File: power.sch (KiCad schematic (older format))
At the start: 18 parts, among them Q1 BSS84, Q2 BSS138, SW1 TL3342, U3 NCP1402SN33T1G

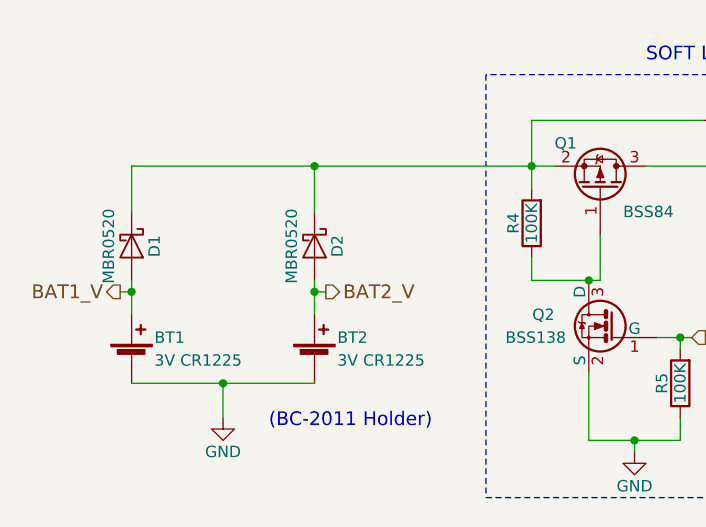
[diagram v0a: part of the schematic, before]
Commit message: attempt 1
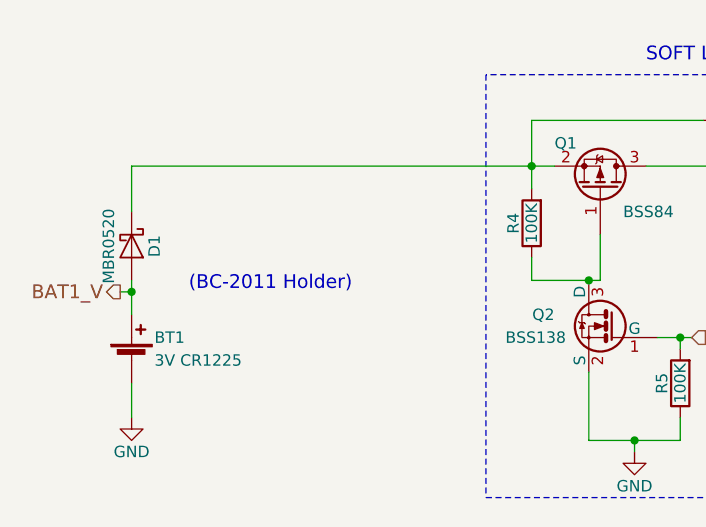
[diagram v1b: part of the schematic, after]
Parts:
- removed BT2: 3V CR1225, BC_2011_CR1225_HOLDER:BC-2011-CR1225, symbol Battery_Cell
- removed D2: MBR0520, Diodes_SMD:D_SOD-123, symbol MBR0520
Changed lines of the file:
@@
-	1    0    0    -1
-$EndComp
-$Comp
-L Battery_Cell BT2
-U 1 1 59A123DB
-P 2300 4050
-F 0 "BT2" H 2400 4150 50  0000 L CNN
-F 1 "3V CR1225" H 2400 4050 50  0000 L CNN
-F 2 "BC_2011_CR1225_HOLDER:BC-2011-CR1225" V 2300 4110 50  0001 C CNN
-F 3 "" V 2300 4110 50  0001 C CNN
-	1    2300 4050
 	1    0    0    -1
 $EndComp
 Wire Wire Line
 	1500 3700 1500 3850
-Wire Wire Line
-	2300 3850 2300 3700
-Wire Wire Line
-	1500 4150 2300 4150
 $Comp
 L GND #PWR014
 U 1 1 59A124B6
-P 1900 4300
-F 0 "#PWR014" H 1900 4050 50  0001 C CNN
-F 1 "GND" H 1900 4150 50  0000 C CNN
-F 2 "" H 1900 4300 50  0001 C CNN
-F 3 "" H 1900 4300 50  0001 C CNN
-	1    1900 4300
-	1    0    0    -1
-$EndComp
-Wire Wire Line
-	1900 4150 1900 4300
-Connection ~ 1900 4150
-Wire Wire Line
-	2300 3400 2300 3200
+P 1500 4300
+F 0 "#PWR014" H 1500 4050 50  0001 C CNN
+F 1 "GND" H 1500 4150 50  0000 C CNN
+F 2 "" H 1500 4300 50  0001 C CNN
+F 3 "" H 1500 4300 50  0001 C CNN
+	1    1500 4300
+	1    0    0    -1
+$EndComp
+Wire Wire Line
+	1500 4150 1500 4300
 Wire Wire Line
 	1500 3200 1500 3400
-Connection ~ 2300 3200
 $Comp
 L SW_Push SW1
@@
 $EndComp
 $Comp
-L MBR0520 D2
-U 1 1 59A17F48
-P 2300 3550
-F 0 "D2" H 2300 3650 50  0000 C CNN
-F 1 "MBR0520" H 2300 3450 50  0000 C CNN
-F 2 "Diodes_SMD:D_SOD-123" H 2300 3375 50  0001 C CNN
-F 3 "" H 2300 3550 50  0001 C CNN
-	1    2300 3550
-	0    1    1    0
-$EndComp
-$Comp
 L GND #PWR015
 U 1 1 59A1839A
@@
 $EndComp
 Wire Wire Line
-	2300 3750 2350 3750
-Connection ~ 2300 3750
-Wire Wire Line
 	1500 3750 1450 3750
 Connection ~ 1500 3750
 Text HLabel 1450 3750 0    60   Output ~ 0
 BAT1_V
-Text HLabel 2350 3750 2    60   Output ~ 0
-BAT2_V
-Text Notes 2100 4350 0    60   ~ 0
+Text Notes 1750 3750 0    60   ~ 0
 (BC-2011 Holder)
 Wire Wire Line
